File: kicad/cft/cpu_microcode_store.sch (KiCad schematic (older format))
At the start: 15 parts, among them U2101 29F040, U2102 29F040, U2103 29F040

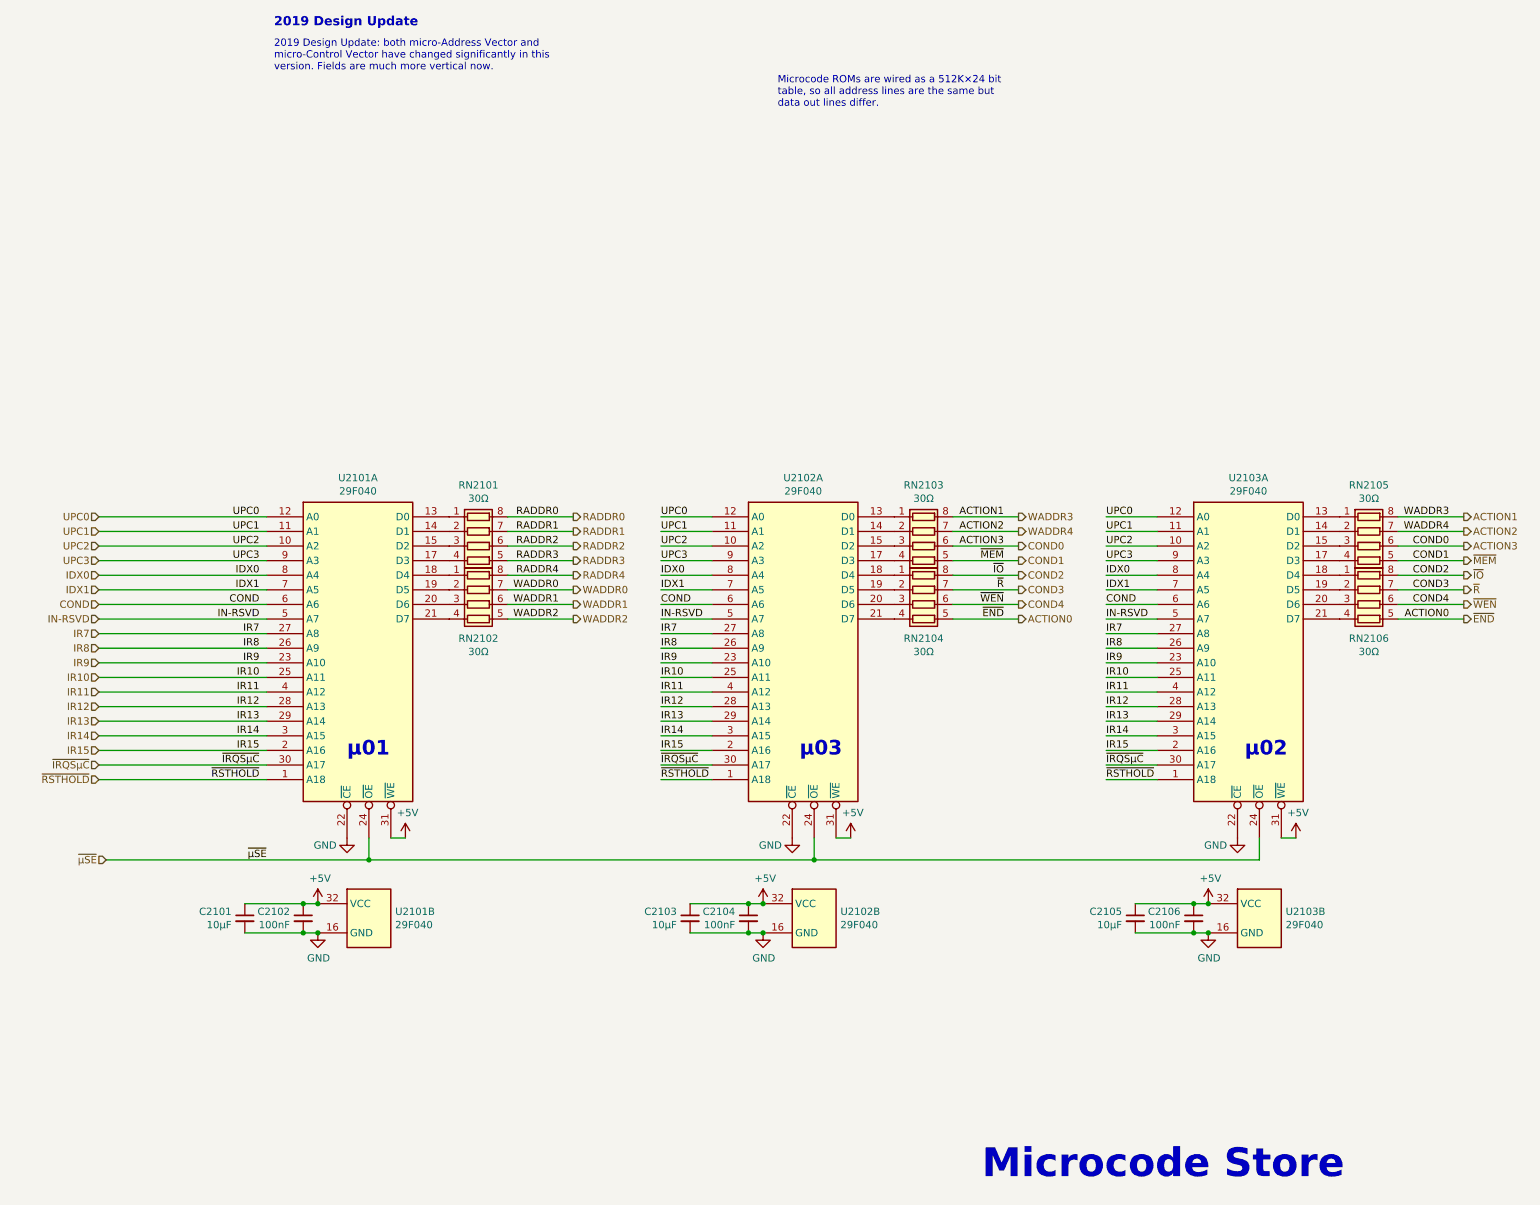
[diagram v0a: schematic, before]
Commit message: Moved things around a bit
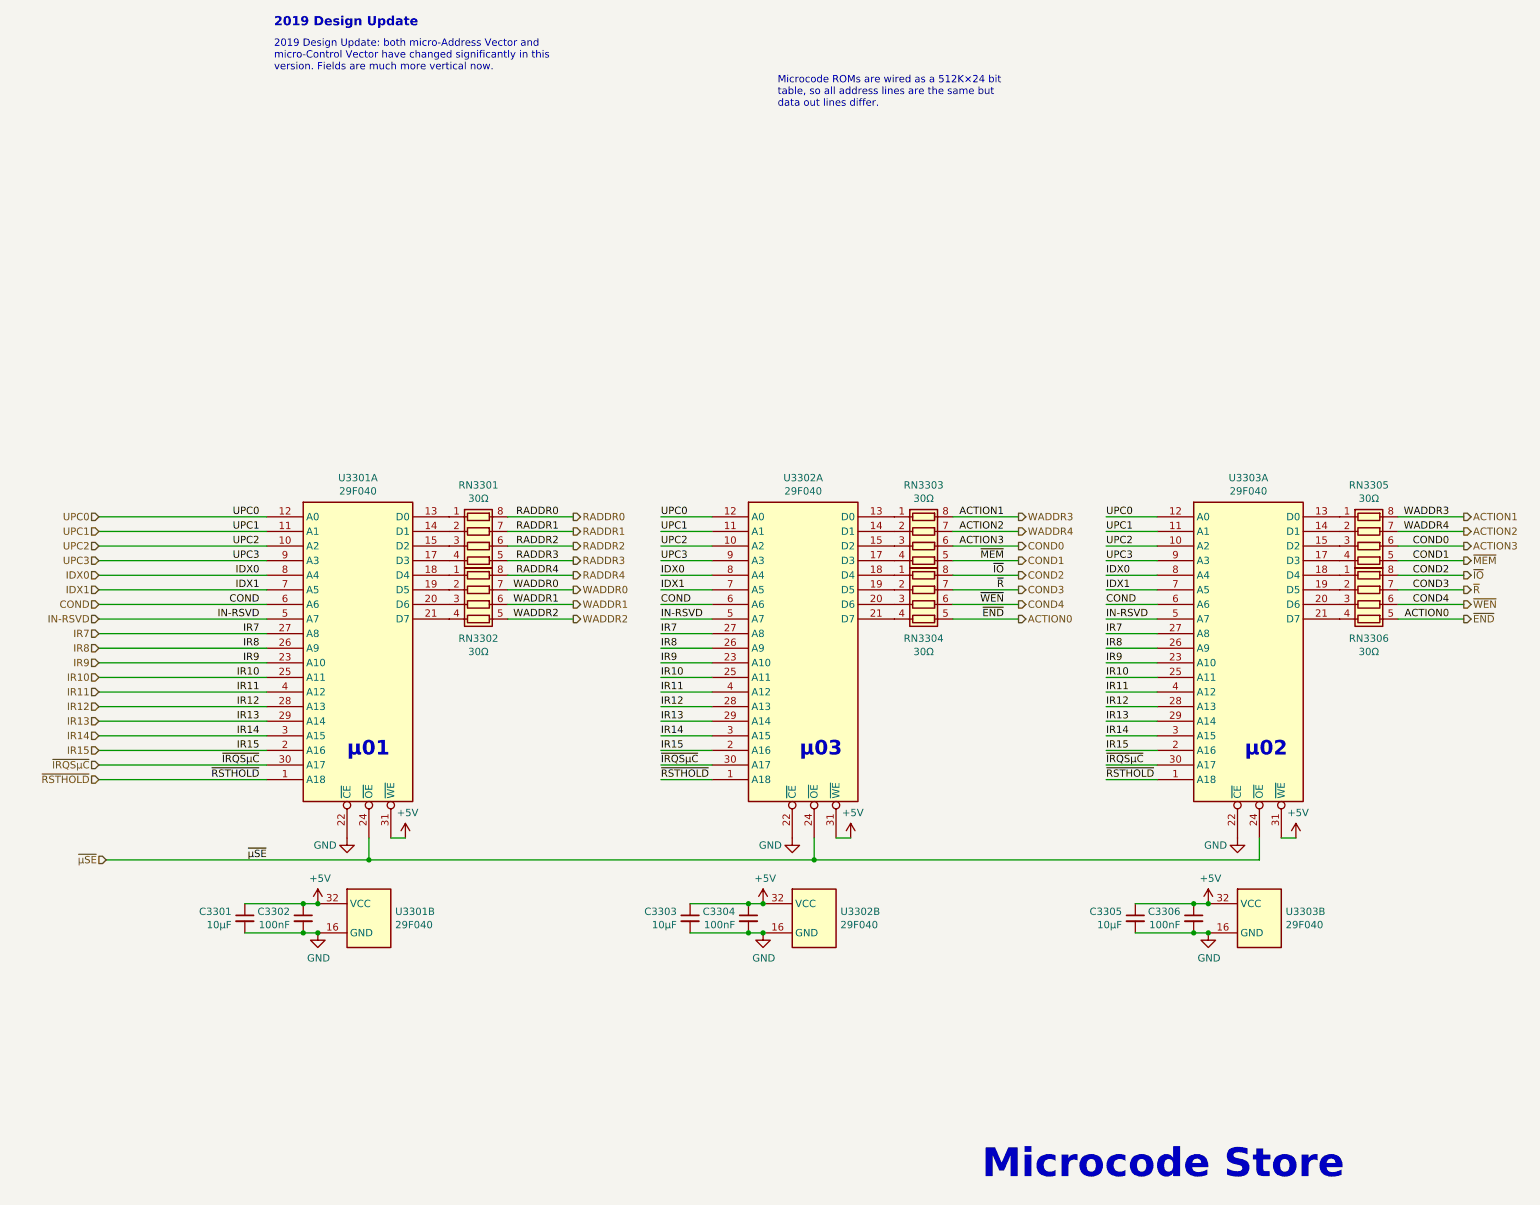
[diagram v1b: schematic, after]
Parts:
- renumbered C2101 to C3301, C2102 to C3302, C2103 to C3303, C2104 to C3304, C2105 to C3305, C2106 to C3306, RN2101 to RN3301, RN2102 to RN3302, RN2103 to RN3303, RN2104 to RN3304, RN2105 to RN3305, RN2106 to RN3306, U2101 to U3301, U2102 to U3302, U2103 to U3303

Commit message: Removed widebus buffer from microcode store µAddr High
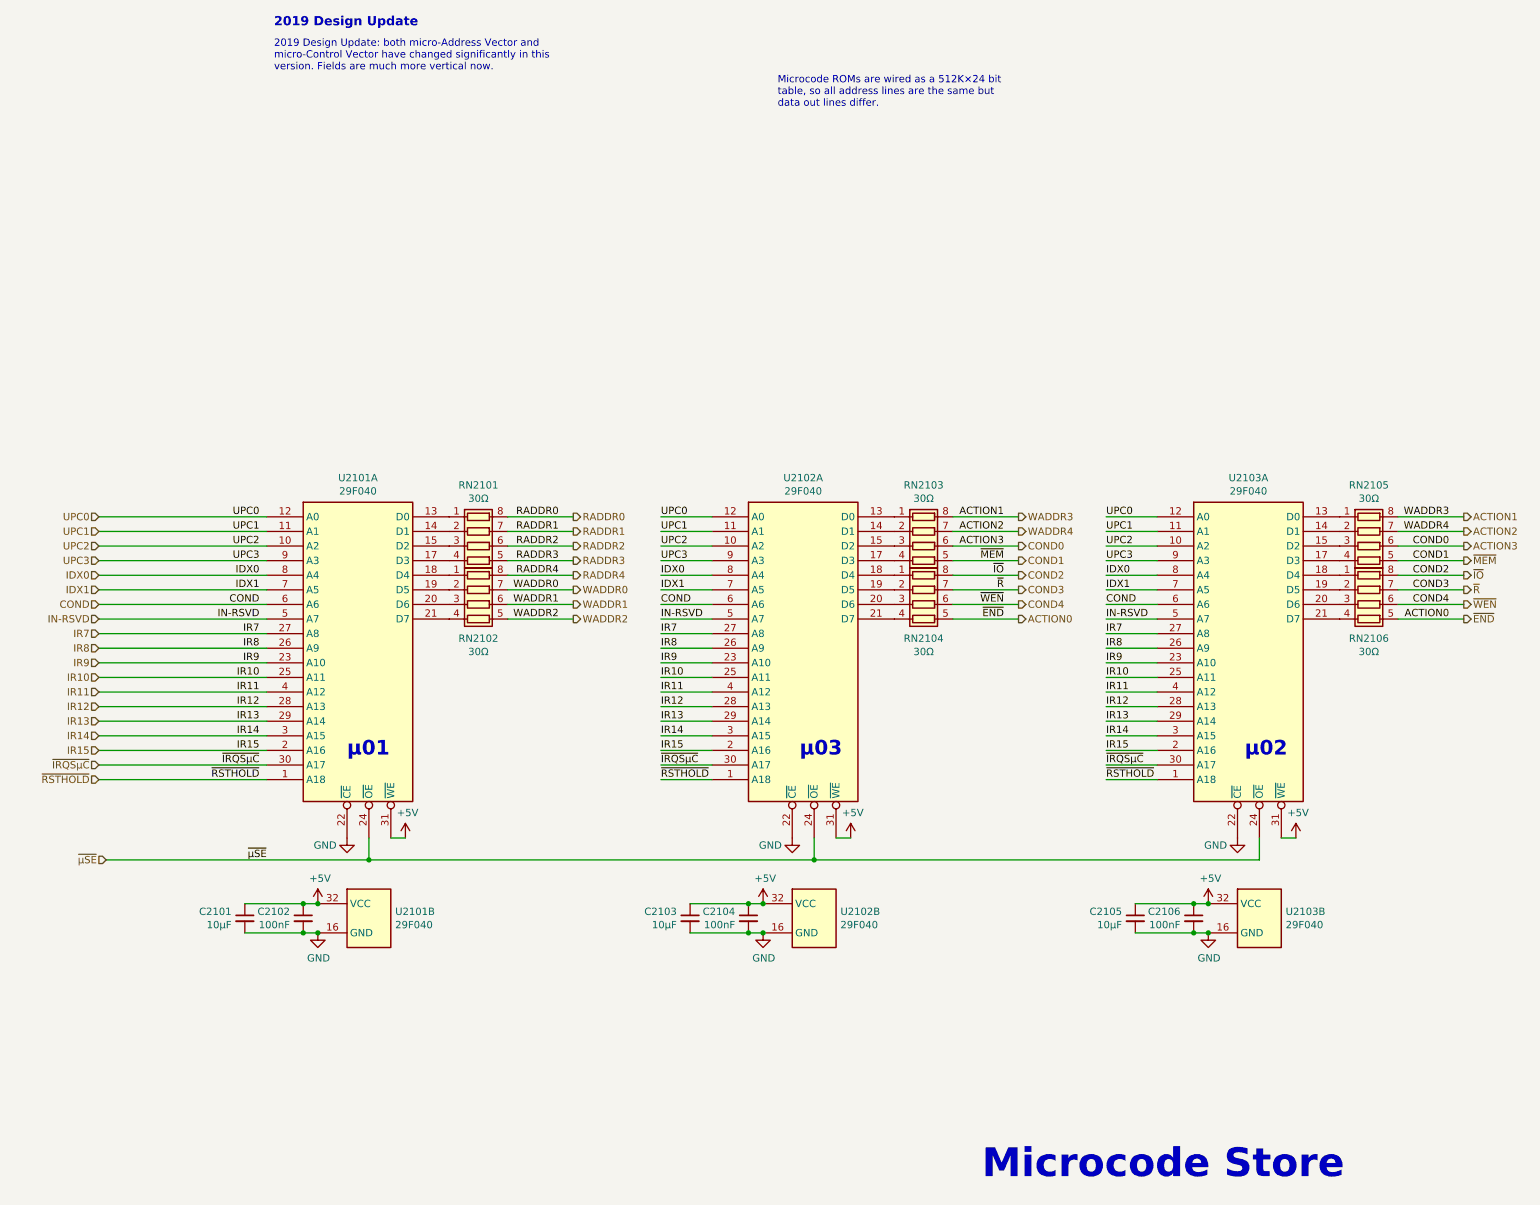
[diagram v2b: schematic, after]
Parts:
- renumbered C3301 to C2101, C3302 to C2102, C3303 to C2103, C3304 to C2104, C3305 to C2105, C3306 to C2106, RN3301 to RN2101, RN3302 to RN2102, RN3303 to RN2103, RN3304 to RN2104, RN3305 to RN2105, RN3306 to RN2106, U3301 to U2101, U3302 to U2102, U3303 to U2103
